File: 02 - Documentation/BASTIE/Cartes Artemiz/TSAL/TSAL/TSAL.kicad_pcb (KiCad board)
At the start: 2 copper layers, 99.1 x 66 mm, 103 parts, among them J1 2P Droit 2-11-2022, J10 2P Droit 2-11-2022, J11 2P Droit 2-11-2022, J2 2P Droit 2-11-2022, J3 2P Droit 2-11-2022, J4 3P Droit 22-11-2032, J5 2P Droit 2-11-2022, J6 2P Droit 2-11-2022, J7 2P Droit 2-11-2022, J8 2P Droit 2-11-2022, J9 2P Droit 2-11-2022, K1 SSR CPC1394GR, K2 SSR CPC1394GR, K3 SSR CPC1394GR, Q2 NMOS SQ2348ES-T1_GE3, Q4 NMOS SQ2348ES-T1_GE3

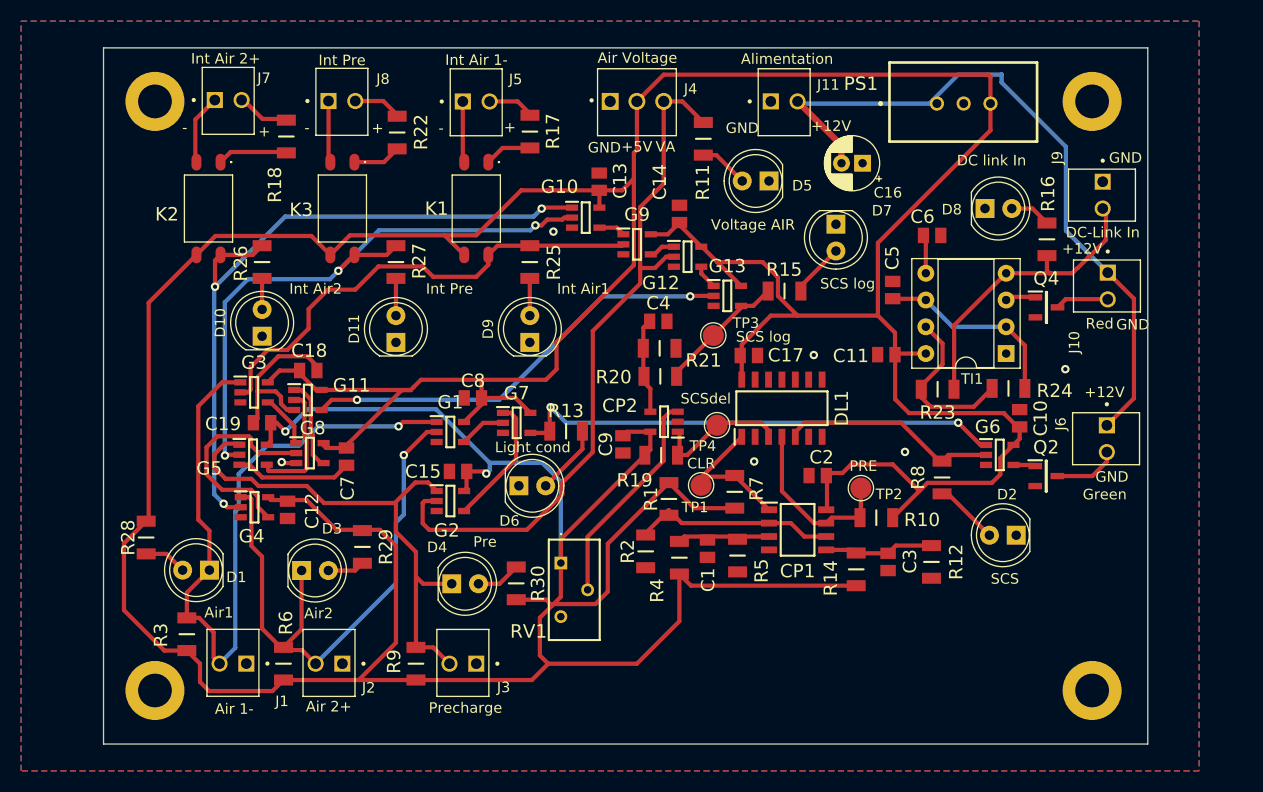
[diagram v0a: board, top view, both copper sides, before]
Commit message: Corrections mineures
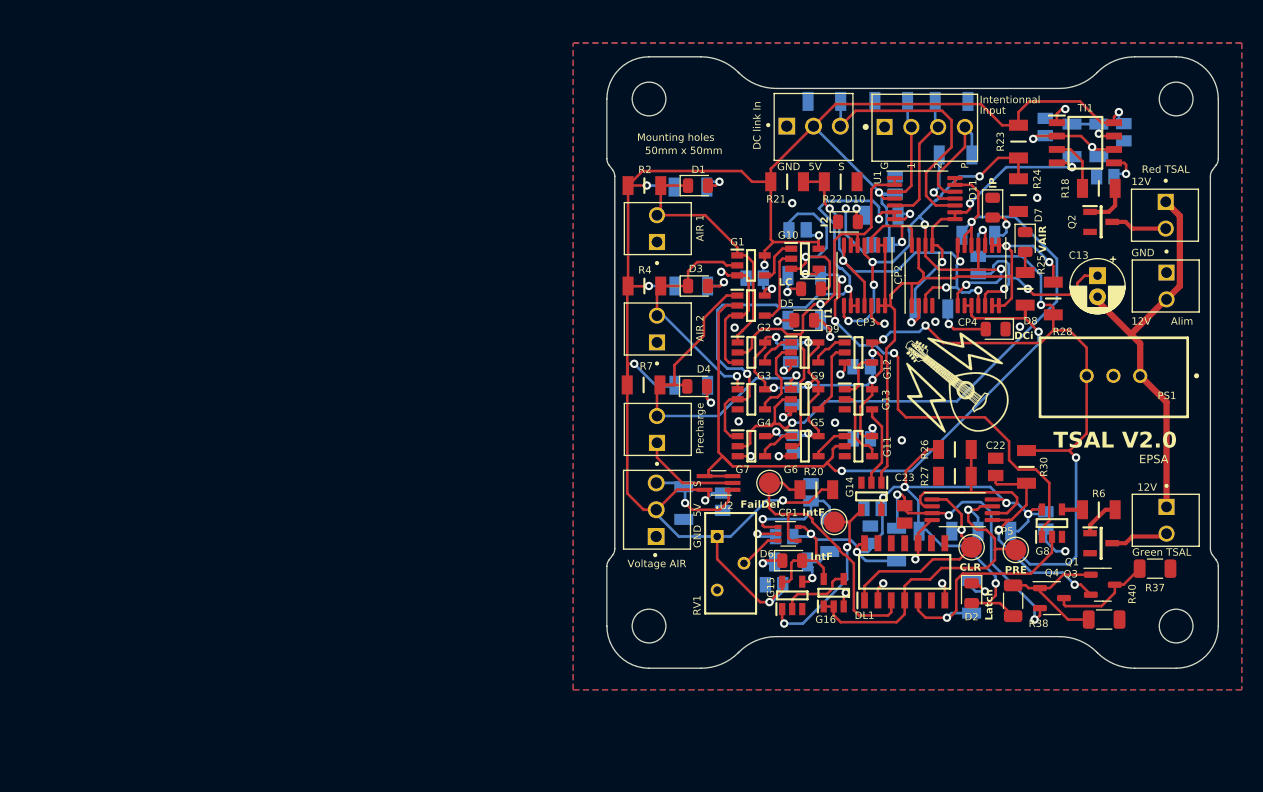
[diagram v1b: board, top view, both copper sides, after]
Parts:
- removed ? (x3): , 
- removed J10, J11: 2P Droit 2-11-2022, EPSA_lib:MOLEX_22-11-2022
- removed K1, K2, K3: SSR CPC1394GR, EPSA_lib:CPC1394GR
- removed REF**: MountingHole_3.2mm_M3_DIN965_Pad, MountingHole:MountingHole_3.2mm_M3_DIN965_Pad
- added C20: 10u, EPSA:CAPC2012X130N, B.Cu at (116.5, 63.0)
- added C21: 2.2u, EPSA:CAPC2012X130N, B.Cu at (118.1, 67.6)
- added C22: 2.2u, EPSA:CAPC2012X130N, F.Cu at (135.6, 65.2)
- added C23: 1u, EPSA:CAPC2012X130N, F.Cu at (127.0, 69.7)
- added CP3: Comparator_Quad, Package_SO:TSSOP-14_4.4x5mm_P0.65mm, F.Cu at (123.2, 47.0)
- added CP4: Comparator_Quad, Package_SO:TSSOP-14_4.4x5mm_P0.65mm, F.Cu at (134.0, 47.0)
- added CP5: Comparator_Dual, Package_SO:TSSOP-8_4.4x3mm_P0.65mm, F.Cu at (132.5, 69.2)
- added G14: Gate AND SN74AHCT1G08DBVR, EPSA:SOT95P280X145-5N, F.Cu at (123.8, 67.9)
- added G15: Gate OR SN74AHCT1G32DBVR, EPSA:SOT95P280X145-5N, F.Cu at (116.3, 77.3)
- added G16: Gate NOR SN74AHCT1G02DBVR, EPSA:SOT95P280X145-5N, F.Cu at (120.3, 77.1)
- added H1: MountingHole, MountingHole:MountingHole_3.2mm_M3, F.Cu at (152.8, 30.2)
- added H2: MountingHole, MountingHole:MountingHole_3.2mm_M3, F.Cu at (102.8, 30.2)
- added H3: MountingHole, MountingHole:MountingHole_3.2mm_M3, F.Cu at (102.8, 80.2)
- added H4: MountingHole, MountingHole:MountingHole_3.2mm_M3, F.Cu at (152.8, 80.2)
- added Q1: NMOS SQ2348ES-T1_GE3, EPSA:SOT95P237X112-3N, F.Cu at (145.6, 72.4)
- added Q3: PMOS SI2343CDS-T1-GE3, Package_TO_SOT_SMD:SOT-23-3, F.Cu at (145.8, 76.3)
- added R31: 500, EPSA:RESC3216X70N, B.Cu at (117.5, 51.2)
- added R32: 500, EPSA:RESC3216X70N, B.Cu at (124.8, 41.3)
- added R33: 5k, EPSA:RESC3216X70N, B.Cu at (135.5, 71.2)
- added R34: 500, EPSA:RESC3216X70N, B.Cu at (134.0, 43.2)
- added R35: 500k, EPSA:RESC3216X70N, B.Cu at (126.2, 72.5)
- added R36: 5k, EPSA:RESC3216X70N, B.Cu at (129.9, 71.2)
- added R37: 1k, Resistor_SMD:R_1206_3216Metric, F.Cu at (150.7, 74.8)
- added R38: 10k, Resistor_SMD:R_1206_3216Metric, F.Cu at (137.3, 77.9)
- added R40: 100k, Resistor_SMD:R_1206_3216Metric, F.Cu at (145.9, 79.6)
- added Ref**: Val**, EPSA:Mandolule Silk, F.Cu at (132.0, 57.1)
- added U1: Opamp_Quad, Package_SO:TSSOP-14_4.4x5mm_P0.65mm, F.Cu at (128.9, 39.7)
- added U2: Opamp, Package_TO_SOT_SMD:SOT-353_SC-70-5_Handsoldering, F.Cu at (109.3, 66.7)
- C1, C10, C11, C12, C14, C17, C18, C2, C3, C4, C5, C6, C7, C8, C9: value Condensateur 0805Y1000104JXT -> 10u; footprint EPSA_lib:CAPC2012X130N -> EPSA:CAPC2012X130N; moved to B.Cu
- C13: value Condensateur 0805Y1000104JXT -> C; footprint EPSA_lib:CAPC2012X130N -> Capacitor_THT:CP_Radial_D5.0mm_P2.00mm
- C15: value Condensateur 0805Y1000104JXT -> 1u; footprint EPSA_lib:CAPC2012X130N -> EPSA:CAPC2012X130N; moved to B.Cu
- C16: value C -> 10u; footprint Capacitor_THT:CP_Radial_D5.0mm_P2.00mm -> EPSA:CAPC2012X130N; moved to B.Cu
- C19: value Condensateur 0805Y1000104JXT -> 0.01u; footprint EPSA_lib:CAPC2012X130N -> EPSA:CAPC2012X130N; moved to B.Cu
- CP1: value Comparateur Double LM393LVDR -> Comparator; footprint EPSA_lib:SOIC127P600X175-8N -> Package_TO_SOT_SMD:SOT-353_SC-70-5
- CP2: value Comparateur TS391ILT -> Comparator_Dual; footprint EPSA_lib:SOT95P280X145-5N -> Package_SO:TSSOP-8_4.4x3mm_P0.65mm
- D1, D10, D11, D2, D3, D4, D5, D6, D7, D8, D9: footprint LED_THT:LED_D5.0mm -> LED_SMD:LED_0805_2012Metric
- DL1: footprint EPSA_lib:SOIC127P600X175-14N -> EPSA:SOIC127P600X175-14N
- G1, G2, G3, G4, G5, G6: footprint EPSA_lib:SOT95P280X145-5N -> EPSA:SOT95P280X145-5N
- G10, G11, G8: value Gate OR SN74AHCT1G32DBVR -> Gate AND SN74AHCT1G08DBVR; footprint EPSA_lib:SOT95P280X145-5N -> EPSA:SOT95P280X145-5N
- G12: value Gate NOR SN74AHCT1G02DBVR -> Gate OR SN74AHCT1G32DBVR; footprint EPSA_lib:SOT95P280X145-5N -> EPSA:SOT95P280X145-5N
- G13: value Gate OR SN74AHCT1G32DBVR -> Gate NOR SN74AHCT1G02DBVR; footprint EPSA_lib:SOT95P280X145-5N -> EPSA:SOT95P280X145-5N
- G7: value Gate AND SN74AHCT1G08DBVR -> Gate OR SN74AHCT1G32DBVR; footprint EPSA_lib:SOT95P280X145-5N -> EPSA:SOT95P280X145-5N
- G9: value Gate NAND SN74AHCT1G00DBVR -> Gate OR SN74AHCT1G32DBVR; footprint EPSA_lib:SOT95P280X145-5N -> EPSA:SOT95P280X145-5N
- J1, J2, J3, J5, J6, J9: footprint EPSA_lib:MOLEX_22-11-2022 -> EPSA:MOLEX_22-11-2022
- J4: footprint EPSA_lib:MOLEX_22-11-2032 -> EPSA:MOLEX_22-11-2032
- J7: value 2P Droit 2-11-2022 -> 4P Droit 22-11-2042; footprint EPSA_lib:MOLEX_22-11-2022 -> EPSA:MOLEX_22-11-2042
- J8: value 2P Droit 2-11-2022 -> 3P Droit 22-11-2032; footprint EPSA_lib:MOLEX_22-11-2022 -> EPSA:MOLEX_22-11-2032
- PS1: footprint EPSA_lib:TSR-2 -> EPSA:TSR-2
- Q2: footprint EPSA_lib:SOT95P237X112-3N -> EPSA:SOT95P237X112-3N
- Q4: value NMOS SQ2348ES-T1_GE3 -> PMOS SI2343CDS-T1-GE3; footprint EPSA_lib:SOT95P237X112-3N -> Package_TO_SOT_SMD:SOT-23-3
- R1, R10, R29, R3, R5, R8, R9: value Résistance RK73H2BLTDD2152F -> 500; footprint EPSA_lib:RESC3216X70N -> EPSA:RESC3216X70N; moved to B.Cu
- R11, R12, R13, R14, R16: value Résistance RK73H2BLTDD2152F -> 500k; footprint EPSA_lib:RESC3216X70N -> EPSA:RESC3216X70N; moved to B.Cu
- R15: value Résistance RK73H2BLTDD2152F -> 2k; footprint EPSA_lib:RESC3216X70N -> EPSA:RESC3216X70N; moved to B.Cu
- R17: value Résistance RK73H2BLTDD2152F -> 200k; footprint EPSA_lib:RESC3216X70N -> EPSA:RESC3216X70N; moved to B.Cu
- R18, R2, R20, R28, R4, R6, R7: value Résistance RK73H2BLTDD2152F -> 10k; footprint EPSA_lib:RESC3216X70N -> EPSA:RESC3216X70N
- R19: value Résistance RK73H2BLTDD2152F -> 390k; footprint EPSA_lib:RESC3216X70N -> EPSA:RESC3216X70N; moved to B.Cu
- R21, R24: value Résistance RK73H2BLTDD2152F -> 12k; footprint EPSA_lib:RESC3216X70N -> EPSA:RESC3216X70N
- R22, R23: value Résistance RK73H2BLTDD2152F -> 82k; footprint EPSA_lib:RESC3216X70N -> EPSA:RESC3216X70N
- R25: value Résistance RK73H2BLTDD2152F -> 500; footprint EPSA_lib:RESC3216X70N -> EPSA:RESC3216X70N
- R26: value Résistance RK73H2BLTDD2152F -> 100k; footprint EPSA_lib:RESC3216X70N -> EPSA:RESC3216X70N
- R27: value Résistance RK73H2BLTDD2152F -> 50k; footprint EPSA_lib:RESC3216X70N -> EPSA:RESC3216X70N
- R30: value Résistance RK73H2BLTDD2152F -> 500k; footprint EPSA_lib:RESC3216X70N -> EPSA:RESC3216X70N
- RV1: footprint EPSA_lib:3296Y1223LF -> EPSA:3296Y1223LF
- TI1: footprint Package_DIP:DIP-8_W7.62mm_Socket -> EPSA:SOIC127P600X175-8N
- TP1, TP2, TP3, TP4: value TestPoint -> type="R" model="TestPoint" lib=""
- moved R28 89.0 mm to (141.1, 49.2)
- moved C19 83.3 mm to (146.0, 37.6)
- moved R6 78.7 mm to (145.4, 69.2), turned to 0 degrees
- moved R18 77.2 mm to (145.4, 38.7), turned to 0 degrees
- moved J5 77.0 mm to (151.8, 68.9), turned to -90 degrees
- moved G8 70.7 mm to (141.0, 70.5), turned to 90 degrees
- moved R26 68.1 mm to (131.8, 63.5), turned to 180 degrees
- moved J7 67.4 mm to (128.9, 32.9)
- moved C15 64.6 mm to (140.3, 32.9), turned to -90 degrees
- moved R3 63.9 mm to (106.7, 38.6), turned to 180 degrees
- moved D1 59.0 mm to (107.4, 38.5), turned to 0 degrees
- moved R29 58.5 mm to (129.5, 50.2), turned to 180 degrees
- moved D11 58.0 mm to (135.3, 40.6), turned to -90 degrees
- moved R27 56.8 mm to (131.8, 66.0), turned to 0 degrees
- moved D10 56.6 mm to (121.6, 41.9), turned to 0 degrees
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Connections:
- C1 pad 1: 0 -> GND
- C1 pad 2: Net-(C1-Pad2) -> +5V
- C10 pad 1: 0 -> GND
- C11 pad 1: 0 -> GND
- C12 pad 1: 0 -> GND
- C13 pad 1: 0 -> GND
- C13 pad 2: +5V -> +12V
- C14 pad 1: 0 -> GND
- C15 pad 1: 0 -> GND
- C15 pad 2: +5V -> Net-(TI1-THRESHOLD)
- C16 pad 1: 0 -> GND
- C16 pad 2: +12V -> +5V
- C17 pad 1: 0 -> GND
- C18 pad 1: 0 -> GND
- C19 pad 1: 0 -> GND
- C19 pad 2: +5V -> Net-(TI1-CONTROL_VOLTAGE)
- C2 pad 1: +5V -> GND
- C2 pad 2: 0 -> +5V
- C3 pad 1: 0 -> GND
- C3 pad 2: Net-(C3-Pad2) -> +5V
- C4 pad 1: Net-(C4-Pad1) -> GND
- C4 pad 2: 0 -> +5V
- C5 pad 1: 0 -> GND
- C5 pad 2: Net-(C5-Pad2) -> +5V
- C6 pad 1: 0 -> GND
- C6 pad 2: Net-(C6-Pad2) -> +5V
- C7 pad 1: 0 -> GND
- C8 pad 1: 0 -> GND
- C9 pad 1: 0 -> GND
- CP1 pad 1: CLR -> Net-(CP1-+)
- CP1 pad 2: mid Pot -> GND
- CP1 pad 3: Net-(C1-Pad2) -> Net-(CP1--)
- CP1 pad 4: 0 -> /Int_del
- CP1 pad 5: Net-(C3-Pad2) -> +5V
- CP2 pad 1: SCS del -> /SCS compliance
- CP2 pad 2: 0 -> /DC-Link_In
- CP2 pad 3: Net-(CP2-Pad3) -> /4.25V
- CP2 pad 4: Net-(C4-Pad1) -> GND
- CP2 pad 5: +5V -> /DC-Link_In
- D1 pad 1: AIR 1 -> /AIR_1
- D1 pad 2: Net-(D1-Pad2) -> Net-(D1-A)
- D10 pad 1: 0 -> GND
- D10 pad 2: Net-(D10-Pad2) -> Net-(D10-A)
- D11 pad 1: 0 -> GND
- D11 pad 2: Net-(D11-Pad2) -> Net-(D11-A)
- D2 pad 1: 0 -> Net-(D2-K)
- D2 pad 2: Net-(D2-Pad2) -> +5V
- D3 pad 1: AIR 2 -> /AIR_2
- D3 pad 2: Net-(D3-Pad2) -> Net-(D3-A)
- D4 pad 1: PreCharge -> /PreCharge
- D4 pad 2: Net-(D4-Pad2) -> Net-(D4-A)
- D5 pad 1: 0 -> GND
- D5 pad 2: Net-(D5-Pad2) -> Net-(D5-A)
- D6 pad 1: 0 -> Net-(D6-K)
- D6 pad 2: Net-(D6-Pad2) -> +5V
- D7 pad 1: 0 -> GND
- D7 pad 2: Net-(D7-Pad2) -> Net-(D7-A)
- D8 pad 1: 0 -> GND
- D8 pad 2: Net-(D8-Pad2) -> Net-(D8-A)
- D9 pad 1: 0 -> GND
- D9 pad 2: Net-(D9-Pad2) -> Net-(D9-A)
- DL1 pad 1: CLR -> /CLR
- DL1 pad 10: 0 -> GND
- DL1 pad 11: 0 -> GND
- DL1 pad 12: 0 -> GND
- DL1 pad 13: 0 -> GND
- DL1 pad 2: 0 -> GND
- DL1 pad 3: SCS del -> /Int_del
- DL1 pad 4: PRE -> /PRE
- DL1 pad 5: SCS -> /INT
- DL1 pad 7: 0 -> GND
- G1 pad 1: AIR 1 -> /AIR_1
- G1 pad 2: AIR 2 -> /AIR_2
- G1 pad 3: 0 -> GND
- G10 pad 1: Int AIR 2 -> Net-(G1-Pad4)
- G10 pad 2: Int PreCharge -> Net-(G10-Pad2)
- G10 pad 3: 0 -> GND
- G10 pad 4: Net-(G10-Pad4) -> /Lightning_cond
- G11 pad 2: Net-(G11-Pad2) -> /VoltageAIR
- G11 pad 3: 0 -> GND
- G12 pad 2: VoltageAIR -> Net-(G12-Pad2)
- G12 pad 3: 0 -> GND
- G13 pad 3: 0 -> GND
- G13 pad 4: SCS log -> Net-(G13-Pad4)
- G2 pad 1: PreCharge -> /PreCharge
- G2 pad 2: VoltageAIR -> /VoltageAIR
- G2 pad 3: 0 -> GND
- G2 pad 4: Net-(G2-Pad4) -> Net-(G10-Pad2)
- G3 pad 1: AIR 1 -> /AIR_1
- G3 pad 2: Int AIR 1 -> /Int_AIR_1
- G3 pad 3: 0 -> GND
- G4 pad 1: AIR 2 -> /AIR_2
- G4 pad 2: Int AIR 2 -> /Int_AIR_2
- G4 pad 3: 0 -> GND
- G5 pad 1: PreCharge -> /PreCharge
- G5 pad 2: Int PreCharge -> /Int_PreCharge
- G5 pad 3: 0 -> GND
- G5 pad 4: Net-(G11-Pad2) -> Net-(G12-Pad2)
- G6 pad 1: Lightning cond -> Net-(G6-Pad1)
- G6 pad 2: SCS -> /Int_AIR_1
- G6 pad 3: 0 -> GND
- G6 pad 4: Net-(G6-Pad4) -> Net-(G11-Pad1)
- G7 pad 1: Net-(G2-Pad4) -> /Int_AIR_2
- G7 pad 2: Net-(G1-Pad4) -> /Int_PreCharge
- G7 pad 3: 0 -> GND
- G7 pad 4: Lightning cond -> Net-(G6-Pad1)
- G8 pad 1: Net-(G3-Pad4) -> /Lightning_cond
- G8 pad 2: Net-(G4-Pad4) -> /INT
- G8 pad 3: 0 -> GND
- G8 pad 4: Net-(G11-Pad1) -> Net-(G8-Pad4)
- G9 pad 1: Net-(G10-Pad4) -> Net-(G3-Pad4)
- G9 pad 2: Int AIR 1 -> Net-(G4-Pad4)
- G9 pad 3: 0 -> GND
- J1 pad 1: 0 -> GND
- J1 pad 2: AIR 1 -> /AIR_1
- J2 pad 1: 0 -> GND
- J2 pad 2: AIR 2 -> /AIR_2
- J3 pad 1: 0 -> GND
- J3 pad 2: PreCharge -> /PreCharge
- J4 pad 1: 0 -> GND
- J4 pad 3: VoltageAIR -> /Raw_VoltageAIR
- J5 pad 1: Net-(J5-Pad1) -> +12V
- J6 pad 1: +12V -> GND
- J6 pad 2: Net-(J6-Pad2) -> +12V
- J7 pad 1: Net-(J7-Pad1) -> GND
- J7 pad 2: Net-(J7-Pad2) -> /Raw_Int_AIR_1
- J8 pad 1: Net-(J8-Pad1) -> GND
- J8 pad 2: Net-(J8-Pad2) -> +5V
- J9 pad 1: 0 -> +12V
- J9 pad 2: DC-Link In -> Net-(J9-Pad2)
- PS1 pad 2: 0 -> GND
- Q2 pad 1: Net-(G6-Pad4) -> Net-(Q2-Pad1)
- Q2 pad 2: 0 -> GND
- Q2 pad 3: Net-(J6-Pad2) -> Net-(J9-Pad2)
- Q4 pad 1: Clign -> Net-(Q3-Pad1)
- Q4 pad 2: 0 -> /dis2
- R1 pad 1: mid Pot -> /INT
- R1 pad 2: +5V -> Net-(D2-K)
- R10 pad 1: PRE -> Net-(G15-Pad4)
- R10 pad 2: +5V -> Net-(D6-K)
- R11 pad 1: Net-(D5-Pad2) -> GND
- R11 pad 2: VoltageAIR -> /Raw_Int_AIR_1
- R12 pad 1: 0 -> GND
- R12 pad 2: Net-(C3-Pad2) -> /Raw_Int_AIR_2
- R13 pad 1: Lightning cond -> GND
- R13 pad 2: Net-(D6-Pad2) -> /Raw_DC-Link_In
- R14 pad 1: Net-(C3-Pad2) -> GND
- R14 pad 2: +5V -> /Raw_Int_PreCharge
- R15 pad 1: SCS log -> Net-(TI1-DISCHARGE)
- R15 pad 2: Net-(D7-Pad2) -> /DC-Link_In
- R16 pad 1: Net-(D8-Pad2) -> GND
- R16 pad 2: DC-Link In -> /Raw_VoltageAIR
- R17 pad 1: Net-(J5-Pad2) -> Net-(TI1-THRESHOLD)
- R17 pad 2: Net-(K1-Pad1) -> Net-(TI1-DISCHARGE)
- R18 pad 1: Net-(J7-Pad2) -> /Clign
- R18 pad 2: Net-(K2-Pad1) -> Net-(Q2-Pad1)
- R19 pad 1: +5V -> Net-(G15-Pad4)
- R19 pad 2: SCS del -> Net-(CP1-+)
- R2 pad 1: 0 -> /AIR_1
- R2 pad 2: mid Pot -> +5V
- R20 pad 1: SCS log -> /Int_del
- R20 pad 2: Net-(C4-Pad1) -> +5V
- R21 pad 1: Net-(C4-Pad1) -> /4.25V
- R21 pad 2: 0 -> +5V
- R22 pad 1: Net-(J8-Pad2) -> GND
- R22 pad 2: Net-(K3-Pad1) -> /4.25V
- R23 pad 1: Net-(R23-Pad1) -> /0.75V
- R23 pad 2: DC-Link In -> +5V
- R24 pad 1: Net-(C5-Pad2) -> GND
- R24 pad 2: Net-(R23-Pad1) -> /0.75V
- R25 pad 1: Int AIR 1 -> Net-(D7-A)
- R25 pad 2: Net-(D9-Pad2) -> /VoltageAIR
- R26 pad 1: Int AIR 2 -> /mid_Pot
- R26 pad 2: Net-(D10-Pad2) -> +5V
- R27 pad 1: Int PreCharge -> GND
- R27 pad 2: Net-(D11-Pad2) -> /mid_Pot
- R28 pad 1: Net-(D1-Pad2) -> +5V
- R28 pad 2: +5V -> /SCS compliance
- R29 pad 1: Net-(D3-Pad2) -> Net-(D8-A)
- R29 pad 2: +5V -> /DC-Link_In
- R3 pad 1: AIR 1 -> Net-(D1-A)
- R30 pad 1: Net-(D4-Pad2) -> /dis1
- R4 pad 1: Net-(C1-Pad2) -> /AIR_2
- R5 pad 1: 0 -> Net-(D3-A)
- R5 pad 2: Net-(C1-Pad2) -> +5V
- R6 pad 1: AIR 2 -> Net-(G8-Pad4)
- R6 pad 2: +5V -> Net-(Q1-Pad1)
- R7 pad 1: CLR -> /PreCharge
- R8 pad 1: SCS -> Net-(D4-A)
- R8 pad 2: Net-(D2-Pad2) -> +5V
- R9 pad 1: PreCharge -> /Lightning_cond
- R9 pad 2: +5V -> Net-(D5-A)
- RV1 pad 2: Net-(CP2-Pad3) -> Net-(CP1--)
- RV1 pad 3: 0 -> GND
- TI1 pad 1: 0 -> GND
- TI1 pad 2: Net-(C5-Pad2) -> Net-(TI1-THRESHOLD)
- TI1 pad 3: Clign -> /Clign
- TI1 pad 4: DC-Link In -> /DC-Link_In
- TI1 pad 5: Net-(C6-Pad2) -> Net-(TI1-CONTROL_VOLTAGE)
- TI1 pad 6: Net-(C5-Pad2) -> Net-(TI1-THRESHOLD)
- TI1 pad 7: Net-(R23-Pad1) -> Net-(TI1-DISCHARGE)
- TP1 pad 1: CLR -> /Int_log
- TP2 pad 1: PRE -> /Int_del
- TP3 pad 1: SCS log -> /PRE
- TP4 pad 1: SCS del -> /CLR
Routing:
- net +5V: track 537.1 -> 403.8 mm, vias 2 -> 33
- net GND: track 0.00 -> 103.8 mm, vias 0 -> 28
- net AIR 1: track 72.2 -> 0.00 mm, vias 1 -> 0
- net /VoltageAIR: track 0.00 -> 72.1 mm, vias 0 -> 2
- net VoltageAIR: track 67.7 -> 0.00 mm
- net Int AIR 2: track 67.3 -> 0.00 mm, vias 3 -> 0
- net /Int_PreCharge: track 0.00 -> 66.3 mm, vias 0 -> 2
- net /SCS compliance: track 0.00 -> 59.4 mm, vias 0 -> 2
- net Int PreCharge: track 58.7 -> 0.00 mm, vias 3 -> 0
- net AIR 2: track 55.5 -> 0.00 mm, vias 1 -> 0
- net PreCharge: track 54.9 -> 0.00 mm
- net /Int_AIR_2: track 0.00 -> 54.3 mm, vias 0 -> 4
- net /0.75V: track 0.00 -> 52.9 mm, vias 0 -> 7
- net Lightning cond: track 46.8 -> 0.00 mm, vias 2 -> 0
- net Int AIR 1: track 45.9 -> 0.00 mm
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- added copper zone on B.Cu, net GND
- added copper zone on F.Cu, net GND
- removed copper zone on B.Cu, net 0
- removed copper zone on F.Cu, net 0
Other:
- board size 99.1 x 66 mm -> 58 x 58 mm
- board text added: "1"
- board text added: "12V"
- board text added: "2"
- board text added: "50mm x 50mm"
- board text added: "5V"
- board text added: "AIR 1"
- board text added: "AIR 2"
- board text added: "Alim"
- board text added: "DCi"
- board text added: "EPSA"
- board text added: "FailDel"
- board text added: "G"
- board text added: "Green TSAL"
- board text added: "I1"
- board text added: "I2"
- board text added: "IP"
- board text added: "Input"
- board text added: "IntF"
- board text added: "Intentionnal"
- board text added: "LC"
- board text added: "Latch"
- board text added: "Mounting holes"
- board text added: "P"
- board text added: "Red TSAL"
- board text added: "S"
- board text added: "TSAL V2.0"
- board text added: "VAIR"
- board text removed: "+"
- board text removed: "+12V"
- board text removed: "+5V"
- board text removed: "-"
- board text removed: "Air 1-"
- board text removed: "Air 2+"
- board text removed: "Air Voltage"
- board text removed: "Air1"
- board text removed: "Air2"
- board text removed: "Alimentation"
- board text removed: "DC-Link In"
- board text removed: "Green"
- board text removed: "Int Air 1-"
- board text removed: "Int Air 2+"
- board text removed: "Int Air1"
- board text removed: "Int Air2"
- board text removed: "Int Pre"
- board text removed: "Light cond"
- board text removed: "Pre"
- board text removed: "Red"
- board text removed: "SCS"
- board text removed: "SCS log"
- board text removed: "SCSdel"
- board text removed: "VA"
